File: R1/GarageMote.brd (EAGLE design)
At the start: 53.3 x 25.7 mm, 16 parts

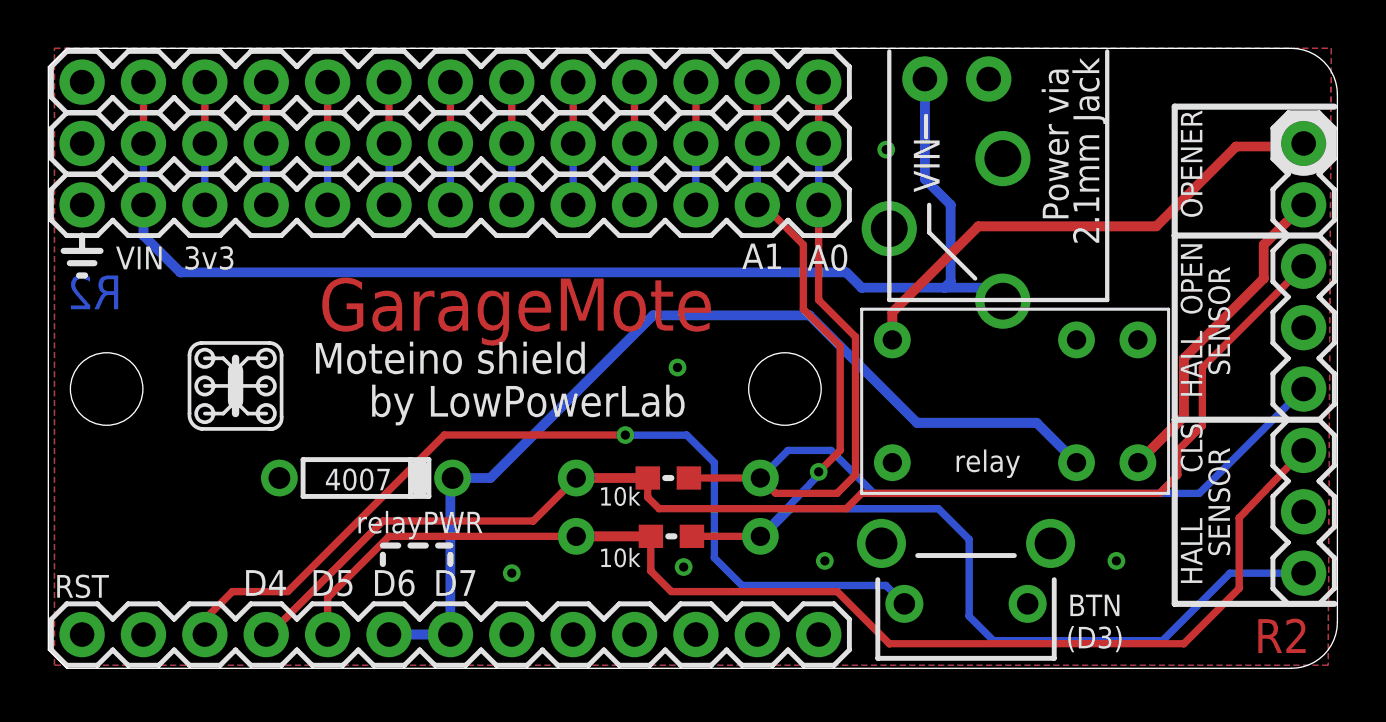
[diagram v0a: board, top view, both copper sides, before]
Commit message: Add R2
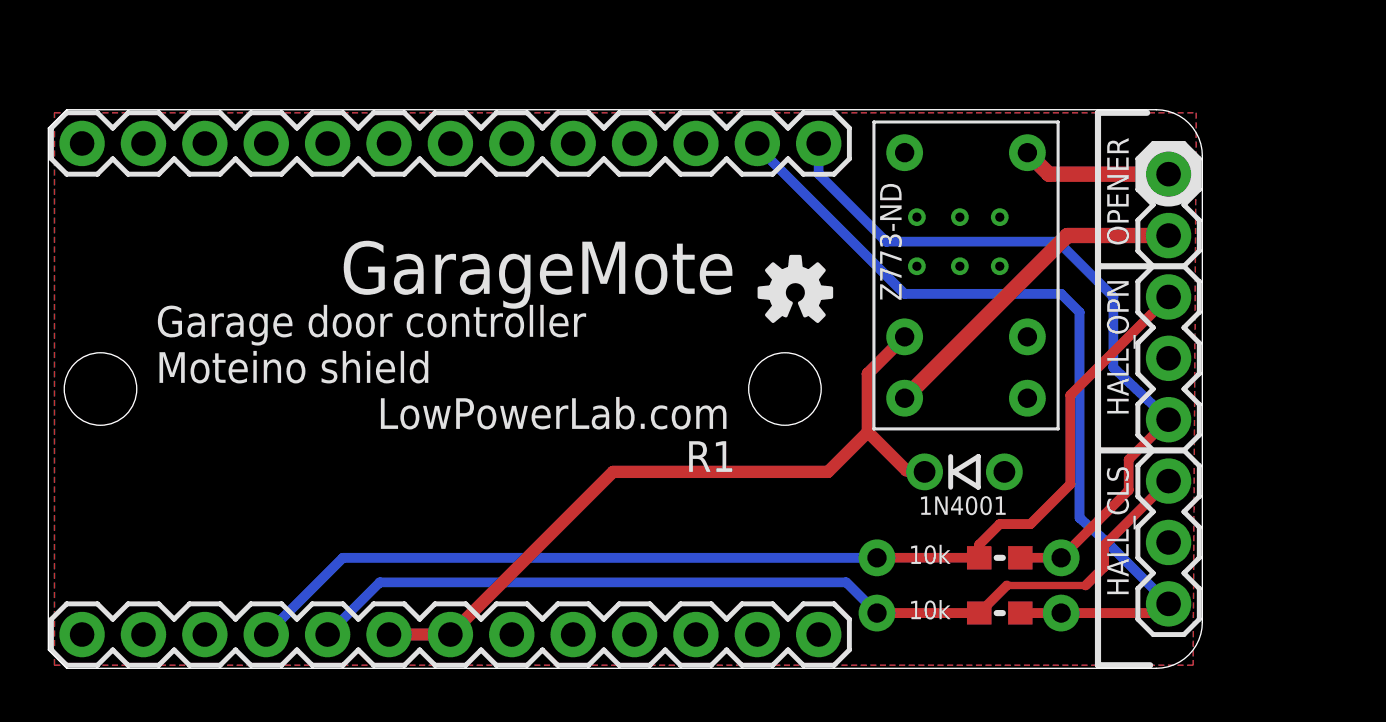
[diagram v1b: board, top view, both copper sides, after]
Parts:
- removed 2.1MM_BARREL_JACK: 2.1MMJACKTH_NOSILK, LowPowerLab:2.1MM_JACK
- removed JP4, JP5: M13, SparkFun-Connectors:1X13
- removed S1: SWITCH-MOMENTARY-2SIDE_EZ, LowPowerLab:TACTILE-PTH-SIDEEZ
- removed U$4: DIODEPTH, LowPowerLab:DIODEPTH
- removed U$5, U$6: (no value), LowPowerLab:LOGO_LOWPOWERLAB
- removed U$9: HDR_2PIN, LowPowerLab:1X02_NS
- added 1N4001: DIODEUPRIGHT, LowPowerLab:DIODE_UPRIGHT
- added U$1, U$2: (no value), SparkFun-Aesthetics:OSHW-LOGO-S
- moved R1 14.1 mm to (39.4, 4.57)
- moved R2 14.0 mm to (39.4, 2.29)
- moved R3 12.9 mm to (38.1, 4.57)
- moved R4 12.8 mm to (38.1, 2.29)
- moved JP3 5.73 mm to (46.4, 20.4)
- moved JRC-2F 5.59 mm to (38.0, 16.3), turned to 90 degrees
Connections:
- removed net N$1: JP2.11, S1.1
- removed net N$10: JP1.11, JP4.11, JP5.11
- removed net N$2: JP1.3, JP4.3, JP5.3
- removed net N$3: JP1.4, JP4.4, JP5.4
- removed net N$4: JP1.5, JP4.5, JP5.5
- removed net N$5: JP1.6, JP4.6, JP5.6
- removed net N$6: JP1.7, JP4.7, JP5.7
- removed net N$7: JP1.8, JP4.8, JP5.8
- removed net N$8: JP1.9, JP4.9, JP5.9
- removed net N$9: JP1.10, JP4.10, JP5.10
- net 5V: no longer 2.1MM_BARREL_JACK.TIP, JP4.2, JP5.2, U$9.1
- net A0: no longer JP4.13, JP5.13
- net A1: no longer JP4.12, JP5.12
- net D6: now also 1N4001.CATHODE_MINUS; no longer U$4.CATHODE_MINUS
- net GND: now also 1N4001.ANODE_PLUS; no longer 2.1MM_BARREL_JACK.RING, JP4.1, JP5.1, S1.2, U$4.ANODE_PLUS, U$9.2
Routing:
- net 5V: track 52.2 -> 0.00 mm
- net N$1: track 37.9 -> 0.00 mm, vias 1 -> 0
- net A0: track 49.8 -> 30.9 mm
- net A1: track 52.7 -> 36.2 mm, vias 1 -> 0
- net RELAYIN: track 21.1 -> 6.21 mm
- net D5: track 50.7 -> 39.0 mm
- net D6: track 40.2 -> 30.9 mm
- net D4: track 52.8 -> 45.6 mm
- net N$9: track 5.08 -> 0.00 mm
- net N$8: track 5.08 -> 0.00 mm
- net N$7: track 5.08 -> 0.00 mm
- net N$6: track 5.08 -> 0.00 mm
- net N$5: track 5.08 -> 0.00 mm
- net N$4: track 5.08 -> 0.00 mm
- net N$3: track 5.08 -> 0.00 mm
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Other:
- board size 53.3 x 25.7 mm -> 47.8 x 23.1 mm
- board text added: "HALL_CLS"
- board text added: "HALL_OPN"
- board text added: "R1"
- board text added: "Z773-ND"
- board text removed: "2.1mm Jack"
- board text removed: "3v3"
- board text removed: "4007"
- board text removed: "BTN (D3)"
- board text removed: "HALL"
- board text removed: "Moteino shield"
- board text removed: "OPEN"
- board text removed: "Power via"
- board text removed: "R2"
- board text removed: "RELAY"
- board text removed: "RST"
- board text removed: "SENSOR"
- board text removed: "VIN"
- board text removed: "XXXXXXXXXXXX"
- board text removed: "by LowPowerLab"
- board text removed: "relay"
- board text removed: "relayPWR"
